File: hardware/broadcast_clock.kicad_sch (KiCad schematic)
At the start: 1 part

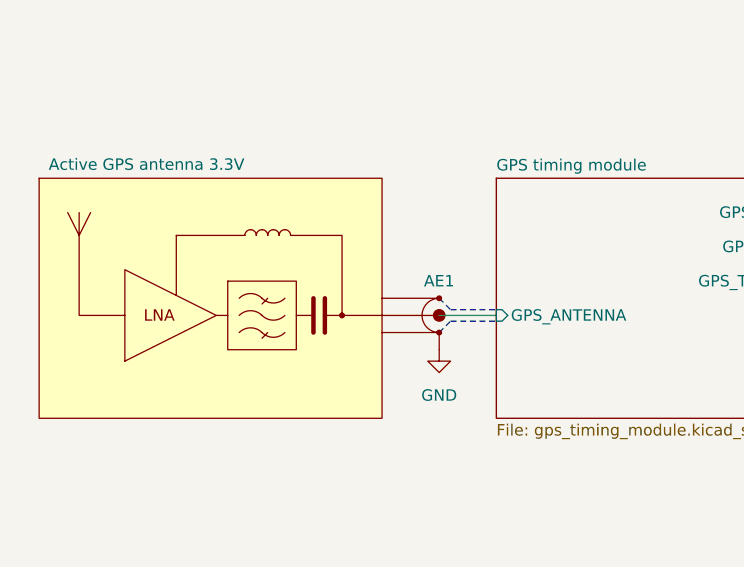
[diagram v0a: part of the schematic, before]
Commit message: Prepare v8 project for KiCAD version 9
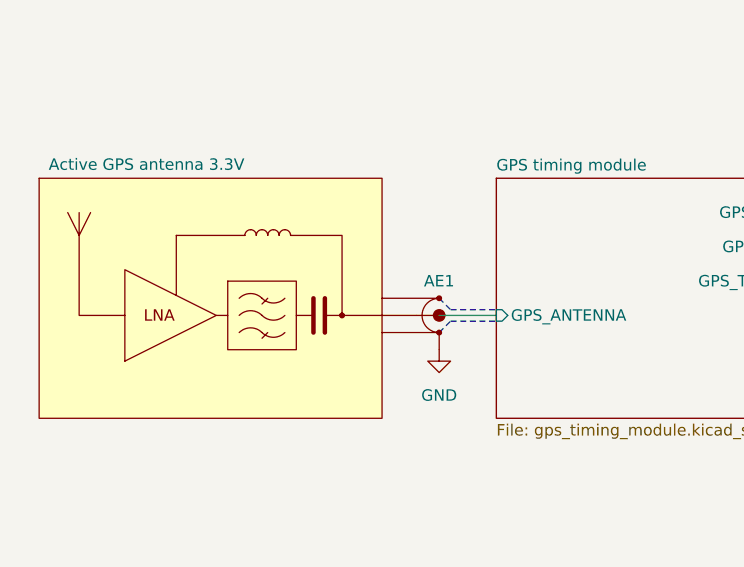
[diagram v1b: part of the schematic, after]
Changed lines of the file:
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@@
 (kicad_sch
-	(version 20231120)
+	(version 20250114)
 	(generator "eeschema")
-	(generator_version "8.0")
+	(generator_version "9.0")
 	(paper "A4")
 	(title_block
@@
 		(at 162.56 49.53)
 		(size 35.56 19.05)
+		(exclude_from_sim no)
+		(in_bom yes)
+		(on_board yes)
+		(dnp no)
 		(fields_autoplaced yes)
 		(stroke
@@
 		(at 210.82 49.53)
 		(size 25.4 90.17)
+		(exclude_from_sim no)
+		(in_bom yes)
+		(on_board yes)
+		(dnp no)
 		(fields_autoplaced yes)
 		(stroke
@@
 		(at 111.76 74.93)
 		(size 38.1 26.67)
+		(exclude_from_sim no)
+		(in_bom yes)
+		(on_board yes)
+		(dnp no)
 		(fields_autoplaced yes)
 		(stroke
@@
 		(at 162.56 74.93)
 		(size 35.56 64.77)
+		(exclude_from_sim no)
+		(in_bom yes)
+		(on_board yes)
+		(dnp no)
 		(fields_autoplaced yes)
 		(stroke
@@
 		)
 	)
+	(embedded_fonts no)
 )
